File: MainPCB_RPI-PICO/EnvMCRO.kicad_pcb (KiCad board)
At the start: 2 copper layers, 109.6 x 69.7 mm, 43 parts, among them SW1 Rotary_Encoder_Switch, U1 Pico

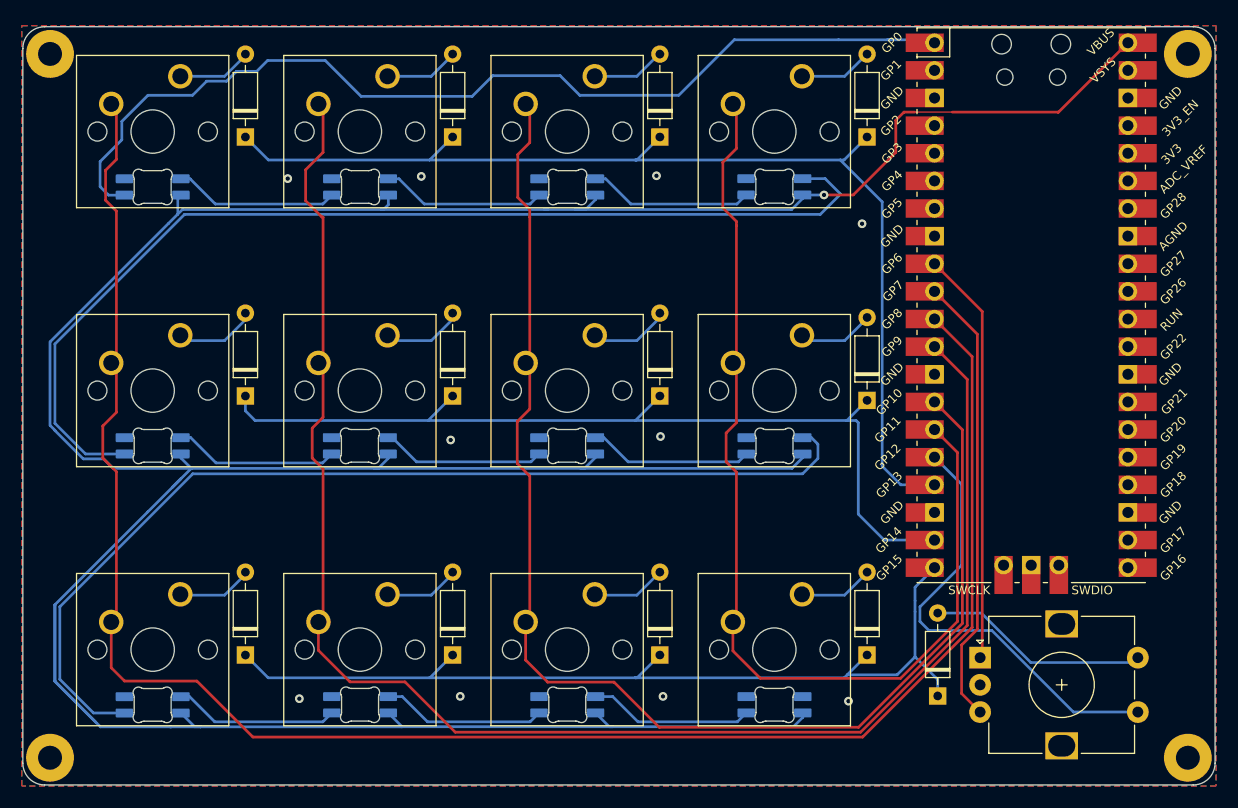
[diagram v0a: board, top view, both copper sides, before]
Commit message: some updates and got rid of other versions, plan to make a XL version in the future that will stay.
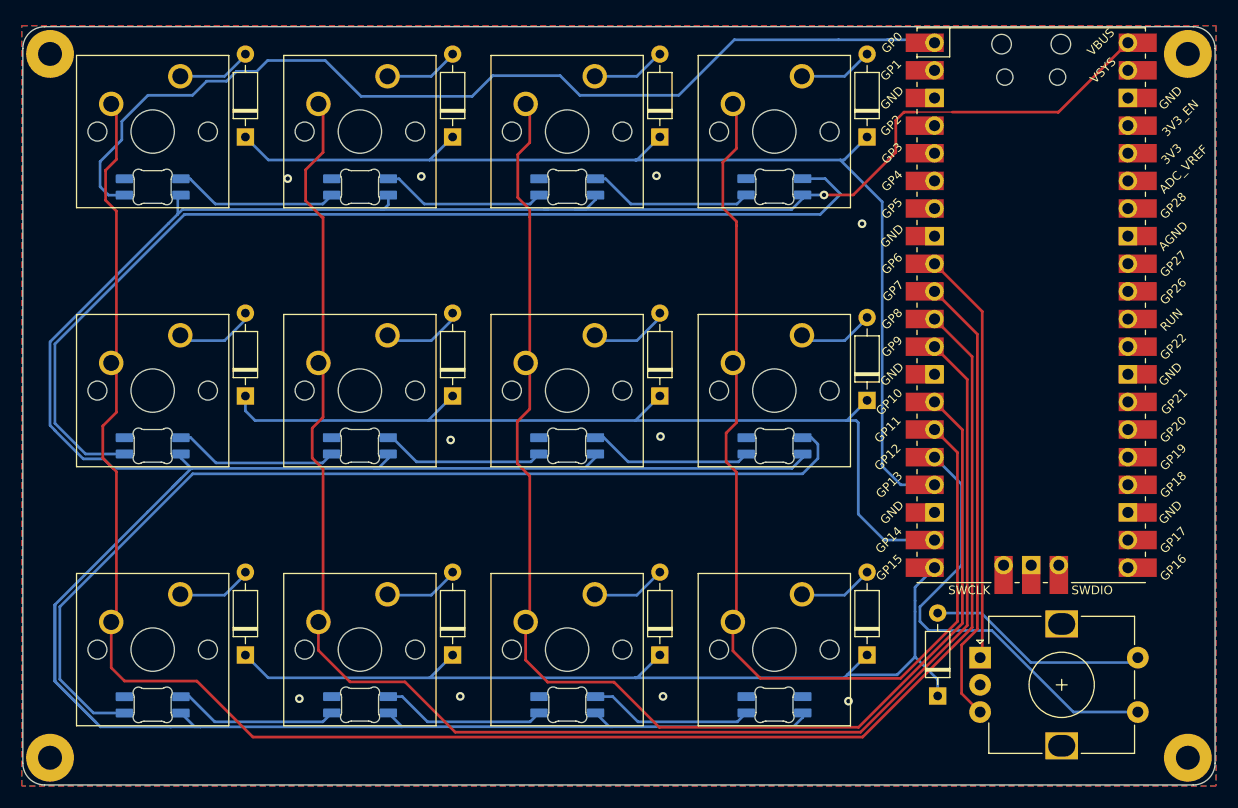
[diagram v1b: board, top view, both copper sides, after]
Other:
- net class Default removed
